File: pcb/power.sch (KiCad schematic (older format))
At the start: 2 parts, among them U1 LTC3456, U100 MCIMX7S5EVM08SC

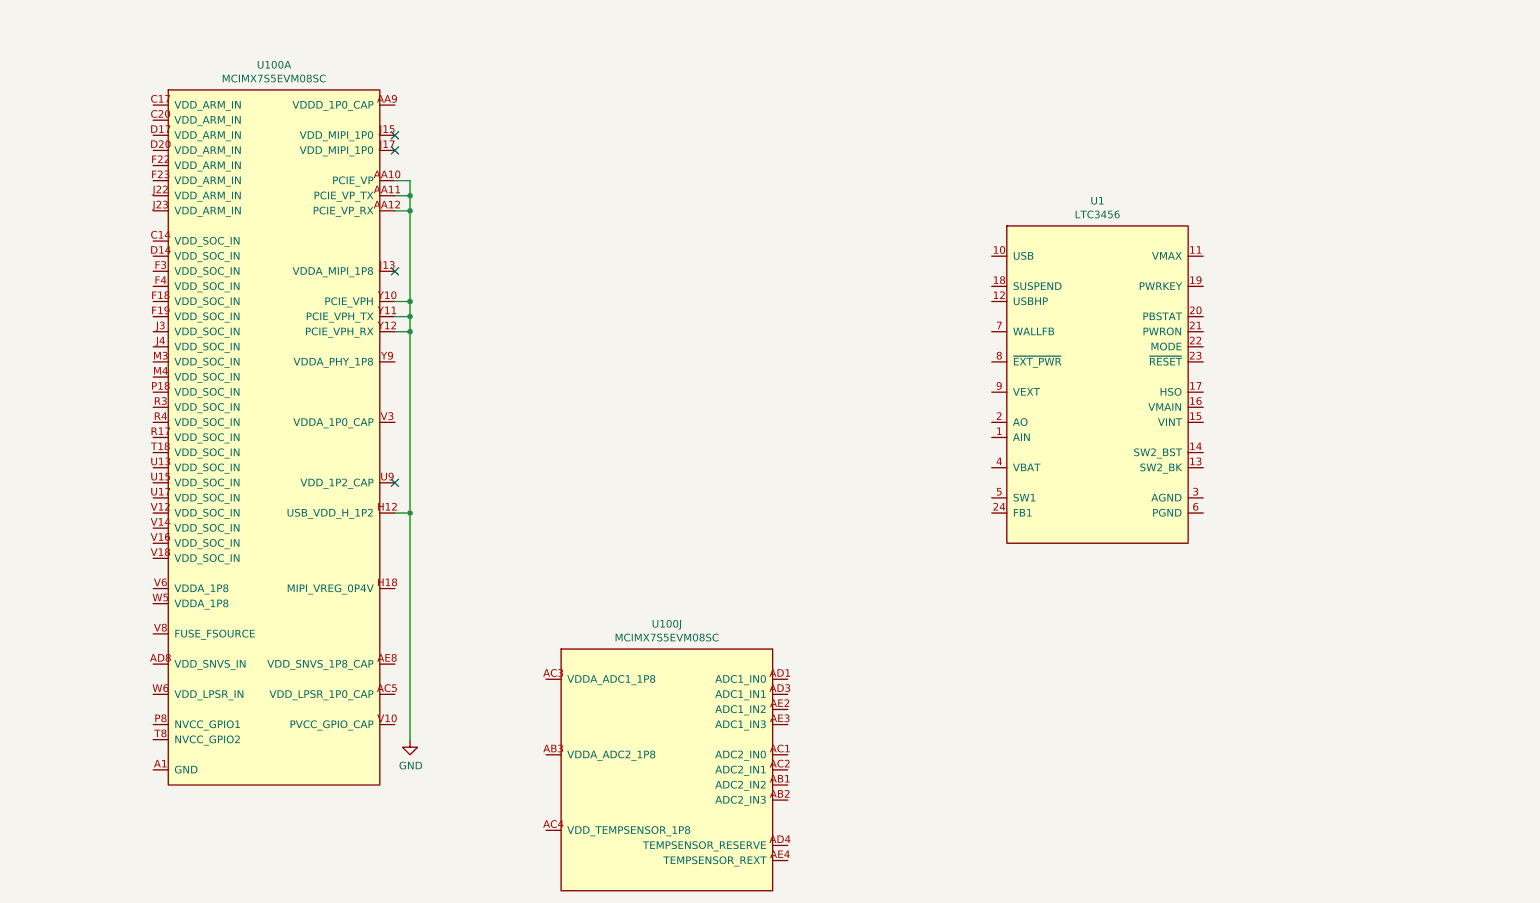
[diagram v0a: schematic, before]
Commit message: pcb: finishing sch for r0.1
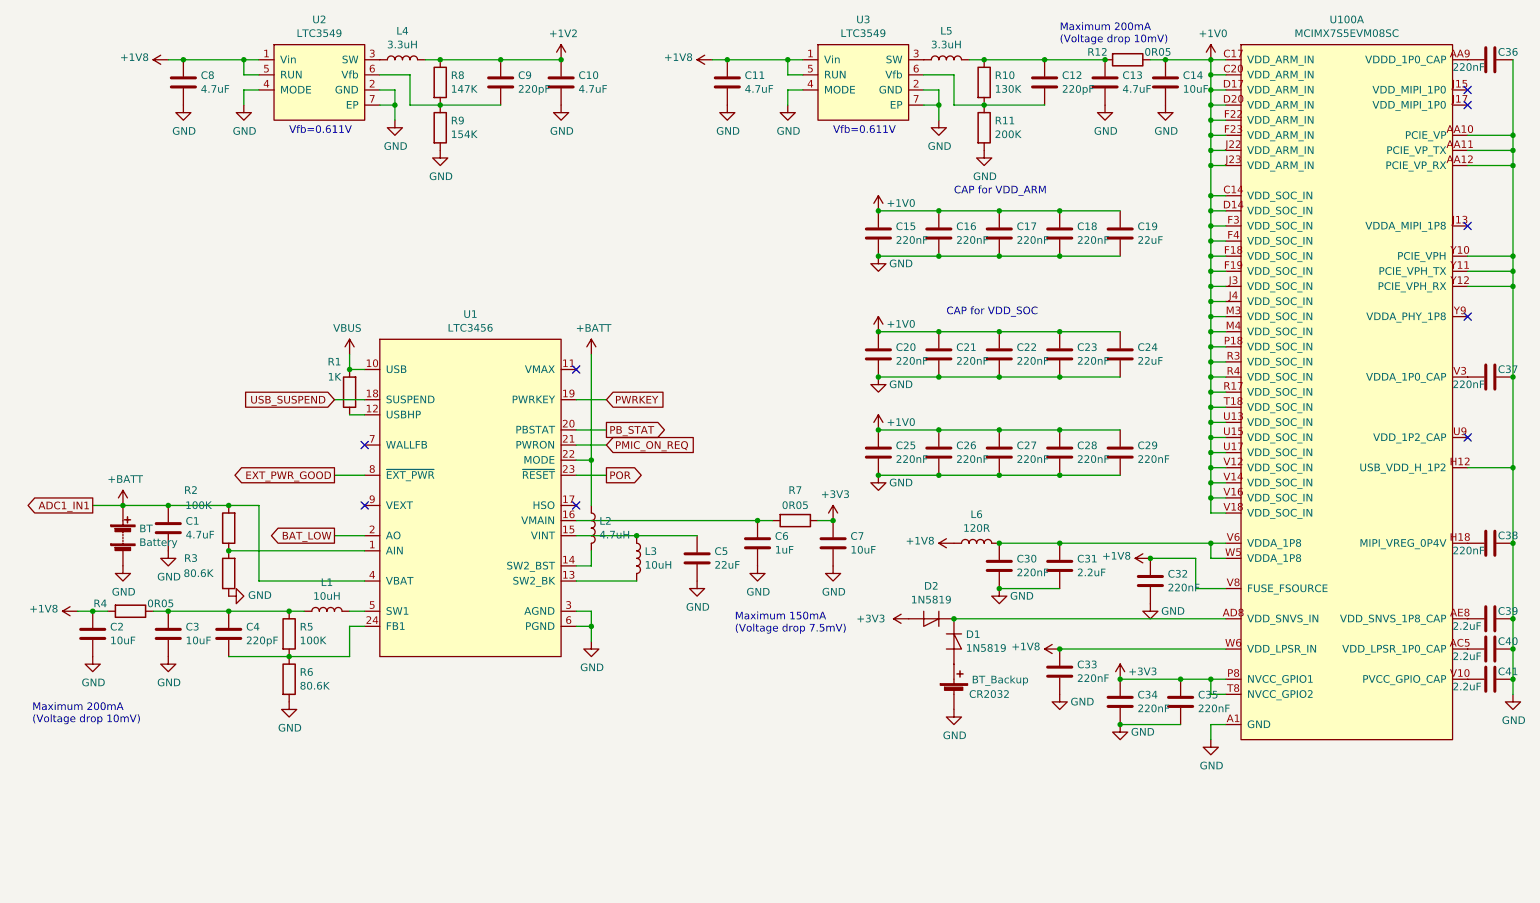
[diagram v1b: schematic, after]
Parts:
- removed unit 10 of U100
- added BT: Battery, Battery:BatteryHolder_Keystone_2468_2xAAA, symbol Device:Battery
- added BT_Backup: CR2032, Battery:BatteryHolder_Keystone_1060_1x2032, symbol Device:Battery_Cell
- added C1, C10, C11, C13, C8: 4.7uF, Capacitor_SMD:C_0603_1608Metric, symbol Device:C
- added C12, C4, C9: 220pF, Capacitor_SMD:C_0402_1005Metric, symbol Device:C
- added C14, C2, C3, C7: 10uF, Capacitor_SMD:C_0603_1608Metric, symbol Device:C
- added C15, C16, C17, C18, C20, C21, C22, C23, C25, C26, C27, C28, C29, C30, C32, C33, C34, C35, C36, C37, C38: 220nF, Capacitor_SMD:C_0402_1005Metric, symbol Device:C
- added C19, C24, C5: 22uF, Capacitor_SMD:C_0603_1608Metric, symbol Device:C
- added C31, C39, C40, C41: 2.2uF, Capacitor_SMD:C_0402_1005Metric, symbol Device:C
- added C6: 1uF, Capacitor_SMD:C_0402_1005Metric, symbol Device:C
- added D1, D2: 1N5819, Diode_SMD:D_SOD-123, symbol Device:D_Shockley
- added L1, L3: 10uH, Inductor_SMD:L_Vishay_IHLP-4040, symbol Device:L
- added L2: 4.7uH, Inductor_SMD:L_Vishay_IHLP-4040, symbol Device:L
- added L4, L5: 3.3uH, Inductor_SMD:L_Vishay_IHLP-4040, symbol Device:L
- added L6: 120R, Inductor_SMD:L_0603_1608Metric, symbol Device:L
- added R1: 1K, Resistor_SMD:R_0603_1608Metric, symbol Device:R
- added R10: 130K, Resistor_SMD:R_0603_1608Metric, symbol Device:R
- added R11: 200K, Resistor_SMD:R_0603_1608Metric, symbol Device:R
- added R12, R4, R7: 0R05, Resistor_SMD:R_1210_3225Metric, symbol Device:R
- added R2, R5: 100K, Resistor_SMD:R_0603_1608Metric, symbol Device:R
- added R3, R6: 80.6K, Resistor_SMD:R_0603_1608Metric, symbol Device:R
- added R8: 147K, Resistor_SMD:R_0603_1608Metric, symbol Device:R
- added R9: 154K, Resistor_SMD:R_0603_1608Metric, symbol Device:R
- added U2, U3: LTC3549, Package_DFN_QFN:DFN-6-1EP_3x2mm_P0.5mm_EP1.65x1.35mm, symbol symbols:LTC3549
- U1: footprint (none) -> Package_DFN_QFN:VQFN-24-1EP_4x4mm_P0.5mm_EP2.45x2.45mm_ThermalVias
- U100: footprint (none) -> footprints:BGA-541_25x25_19.0x19.0mm
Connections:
- net GND: now also U1.3 (AGND), U1.6 (PGND), U100.A1 (GND), U100.A13 (GND), U100.A17 (GND), U100.A21 (GND), U100.A25 (GND), U100.A3 (GND), U100.A6 (GND), U100.A9 (GND), U100.AA1 (GND), U100.AA15 (GND), U100.AA2 (GND), U100.AA23 (GND), U100.AA6 (GND), U100.AA8 (GND), U100.AB12 (GND), U100.AB4 (GND), U100.AB5 (GND), U100.AB7 (GND), U100.AB9 (GND), U100.AC12 (GND), U100.AC15 (GND), U100.AC17 (GND), U100.AC19 (GND), U100.AC21 (GND), U100.AC23 (GND), U100.AC6 (GND), U100.AC9 (GND), U100.AD12 (GND), U100.AD2 (GND), U100.AD5 (GND), U100.AD7 (GND), U100.AD9 (GND), U100.AE1 (GND), U100.AE12 (GND), U100.AE24 (GND), U100.AE25 (GND), U100.AE5 (GND), U100.AE7 (GND), U100.AE9 (GND), U100.B13 (GND), U100.B17 (GND), U100.B21 (GND), U100.B3 (GND), U100.B6 (GND), U100.B9 (GND), U100.C13 (GND), U100.C15 (GND), U100.C16 (GND), U100.C18 (GND), U100.C19 (GND), U100.C9 (GND), U100.D1 (GND), U100.D10 (GND), U100.D2 (GND), U100.D22 (GND), U100.D4 (GND), U100.D7 (GND), U100.F11 (GND), U100.F13 (GND), U100.F7 (GND), U100.F8 (GND), U100.G11 (GND), U100.G13 (GND), U100.G15 (GND), U100.G17 (GND), U100.G19 (GND), U100.G22 (GND), U100.G4 (GND), U100.G7 (GND), U100.G9 (GND), U100.H1 (GND), U100.H2 (GND), U100.J19 (GND), U100.J7 (GND), U100.K10 (GND), U100.K12 (GND), U100.K14 (GND), U100.K16 (GND), U100.K22 (GND), U100.K4 (GND), U100.L11 (GND), U100.L13 (GND), U100.L15 (GND), U100.L19 (GND), U100.L7 (GND), U100.M10 (GND), U100.M12 (GND), U100.M14 (GND), U100.M16 (GND), U100.M24 (GND), U100.M25 (GND), U100.N11 (GND), U100.N13 (GND), U100.N15 (GND), U100.N19 (GND), U100.N4 (GND), U100.N7 (GND), U100.P10 (GND), U100.P12 (GND), U100.P14 (GND), U100.P16 (GND), U100.R11 (GND), U100.R13 (GND), U100.R15 (GND), U100.R19 (GND), U100.R20 (GND), U100.R21 (GND), U100.R23 (GND), U100.R7 (GND), U100.T10 (GND), U100.T12 (GND), U100.T14 (GND), U100.T16 (GND), U100.T20 (GND), U100.T4 (GND), U100.U11 (GND), U100.U19 (GND), U100.U20 (GND), U100.U23 (GND), U100.U7 (GND), U100.V20 (GND), U100.W1 (GND), U100.W11 (GND), U100.W13 (GND), U100.W15 (GND), U100.W17 (GND), U100.W19 (GND), U100.W2 (GND), U100.W20 (GND), U100.W23 (GND), U100.W4 (GND), U100.W7 (GND), U100.W9 (GND), U100.Y13 (GND), U100.Y14 (GND), U100.Y15 (GND), U100.Y16 (GND), U100.Y17 (GND), U100.Y18 (GND), U100.Y19 (GND), U100.Y6 (GND), BT.2 (-), BT_Backup.2 (-), C1.2, C10.2, C11.2, C13.2, C14.2, C15.2, C16.2, C17.2, C18.2, C19.2, C2.2, C20.2, C21.2, C22.2, C23.2, C24.2, C25.2, C26.2, C27.2, C28.2, C29.2, C3.2, C30.2, C31.2, C32.2, C33.2, C34.2, C35.2, C36.1, C37.1, C38.1, C39.1, C40.1, C41.1, C5.2, C6.2, C7.2, C8.2, R11.2, R3.1, R6.2, R9.2, U2.2 (GND), U2.4 (MODE), U2.7 (EP), U3.2 (GND), U3.4 (MODE), U3.7 (EP)
- net at U100.AA9 (VDDD_1P0_CAP): now also C36.2
- net at U100.AC5 (VDD_LPSR_1P0_CAP): now also C40.2
- net at U100.AD8 (VDD_SNVS_IN): now also D1.1 (K), D2.1 (K)
- net at U100.AE8 (VDD_SNVS_1P8_CAP): now also C39.2
- net +1V0: now reaches U100.C14 (VDD_SOC_IN)
- net +1V0: now also U100.C17 (VDD_ARM_IN), U100.C20 (VDD_ARM_IN), U100.D14 (VDD_SOC_IN), U100.D17 (VDD_ARM_IN), U100.D20 (VDD_ARM_IN), U100.F18 (VDD_SOC_IN), U100.F19 (VDD_SOC_IN), U100.F22 (VDD_ARM_IN), U100.F23 (VDD_ARM_IN), U100.F3 (VDD_SOC_IN), U100.F4 (VDD_SOC_IN), U100.J22 (VDD_ARM_IN), U100.J23 (VDD_ARM_IN), U100.J3 (VDD_SOC_IN), U100.J4 (VDD_SOC_IN), U100.M3 (VDD_SOC_IN), U100.M4 (VDD_SOC_IN), U100.P18 (VDD_SOC_IN), U100.R17 (VDD_SOC_IN), U100.R3 (VDD_SOC_IN), U100.R4 (VDD_SOC_IN), U100.T18 (VDD_SOC_IN), U100.U13 (VDD_SOC_IN), U100.U15 (VDD_SOC_IN), U100.U17 (VDD_SOC_IN), U100.V12 (VDD_SOC_IN), U100.V14 (VDD_SOC_IN), U100.V16 (VDD_SOC_IN), U100.V18 (VDD_SOC_IN), C14.1, C15.1, C16.1, C17.1, C18.1, C19.1, C20.1, C21.1, C22.1, C23.1, C24.1, C25.1, C26.1, C27.1, C28.1, C29.1, R12.1
- net at U100.H18 (MIPI_VREG_0P4V): now also C38.2
- net +3V3: now reaches U100.P8 (NVCC_GPIO1)
- net +3V3: now also U100.T8 (NVCC_GPIO2), C34.1, C35.1, C7.1, D2.2 (A), R7.1
- net at U100.V10 (PVCC_GPIO_CAP): now also C41.2
- net at U100.V3 (VDDA_1P0_CAP): now also C37.2
- net at U100.V6 (VDDA_1P8): now also U100.W5 (VDDA_1P8), C30.1, C31.1, L6.2
- net +1V8: now reaches U100.V8 (FUSE_FSOURCE)
- net +1V8: now also U100.W6 (VDD_LPSR_IN), C11.1, C2.1, C32.1, C33.1, C8.1, L6.1, R4.2, U2.1 (Vin), U2.5 (RUN), U3.1 (Vin), U3.5 (RUN)
- net at U1.1 (AIN): now also R2.1, R3.2
- net VBUS: now reaches U1.10 (USB)
- net VBUS: now also R1.2
- net at U1.12 (USBHP): now also R1.1
- net at U1.13 (SW2_BK): now also L3.2
- net at U1.14 (SW2_BST): now also L2.2
- net at U1.15 (VINT): now also C5.1, L3.1
- net at U1.16 (VMAIN): now also C6.1, R7.2
- net USB_SUSPEND: now reaches U1.18 (SUSPEND)
- net PWRKEY: now reaches U1.19 (PWRKEY)
- net BAT_LOW: now reaches U1.2 (AO)
- net PB_STAT: now reaches U1.20 (PBSTAT)
- net PMIC_ON_REQ: now reaches U1.21 (PWRON)
- net +BATT: now reaches U1.22 (MODE)
- net +BATT: now also U1.4 (VBAT), BT.1 (+), C1.1, L2.1, R2.2
- net POR: now reaches U1.23 (~RESET)
- net at U1.24 (FB1): now also C4.2, R5.2, R6.1
- net at U1.5 (SW1): now also L1.2
- net EXT_PWR_GOOD: now reaches U1.8 (~EXT_PWR)
- new net: C3.1, C4.1, L1.1, R4.1, R5.1
- new net: L5.1, U3.3 (SW)
- new net: C12.2, R10.2, R11.1, U3.6 (Vfb)
- new net: C12.1, C13.1, L5.2, R10.1, R12.2
- new net: L4.1, U2.3 (SW)
- new net: C9.2, R8.2, R9.1, U2.6 (Vfb)
- new net: BT_Backup.1 (+), D1.2 (A)
- new net +1V2: C10.1, C9.1, L4.2, R8.1
- no-connect marks 4 -> 9
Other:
- note added: "CAP for VDD_ARM"
- note added: "CAP for VDD_SOC"
- note added: "Maximum 150mA\n(Voltage drop 7.5mV)"
- note added: "Maximum 200mA\n(Voltage drop 10mV)"
- note added: "Vfb=0.611V"
- moved on the sheet: U1, U100A
